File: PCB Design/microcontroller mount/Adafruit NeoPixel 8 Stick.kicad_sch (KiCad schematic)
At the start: 2 parts, among them CN2 1X4SMT, U1 DFR0282

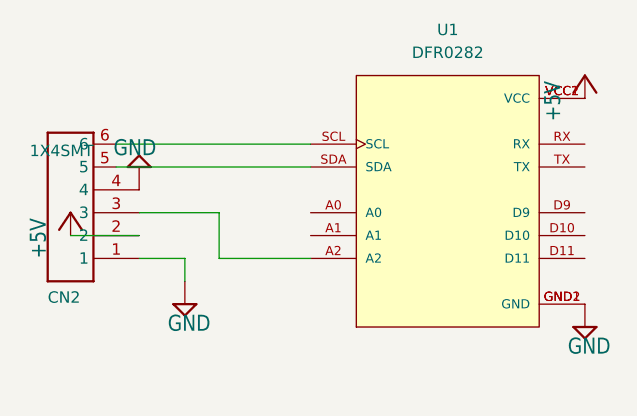
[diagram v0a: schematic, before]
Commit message: updates
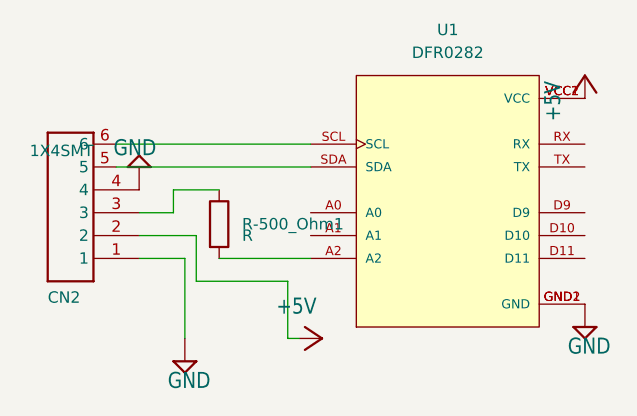
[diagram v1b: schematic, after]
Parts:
- added R-500_Ohm1: R, Resistor_THT:R_Axial_DIN0204_L3.6mm_D1.6mm_P7.62mm_Horizontal, symbol Device:R
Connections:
- net at CN2.3: now also R-500_Ohm1.1; no longer U1.A2
- new net: R-500_Ohm1.2, U1.A2
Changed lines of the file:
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@@
 (kicad_sch (version 20211123) (generator eeschema)
   (paper "A4")
+  (wire (pts (xy 46.99 129.54) (xy 57.15 129.54))
+    (stroke (width 0) (type default) (color 0 0 0 0))
+  )
   (wire (pts (xy 40.64 127) (xy 45.72 127))
     (stroke (width 0) (type default) (color 0 0 0 0))
   )
-  (wire (pts (xy 45.72 127) (xy 45.72 129.54))
-    (stroke (width 0) (type default) (color 0 0 0 0))
-  )
   (wire (pts (xy 38.1 116.84) (xy 59.69 116.84))
     (stroke (width 0) (type default) (color 0 0 0 0))
   )
+  (wire (pts (xy 44.45 119.38) (xy 44.45 121.92))
+    (stroke (width 0) (type default) (color 0 0 0 0))
+  )
+  (wire (pts (xy 49.53 119.38) (xy 44.45 119.38))
+    (stroke (width 0) (type default) (color 0 0 0 0))
+  )
   (wire (pts (xy 38.1 114.3) (xy 59.69 114.3))
     (stroke (width 0) (type default) (color 0 0 0 0))
   )
-  (wire (pts (xy 49.53 121.92) (xy 40.64 121.92))
-    (stroke (width 0) (type default) (color 0 0 0 0))
-  )
-  (wire (pts (xy 49.53 127) (xy 49.53 121.92))
-    (stroke (width 0) (type default) (color 0 0 0 0))
-  )
-  (wire (pts (xy 59.69 127) (xy 49.53 127))
-    (stroke (width 0) (type default) (color 0 0 0 0))
-  )
-  (wire (pts (xy 33.02 124.46) (xy 40.64 124.46))
+  (wire (pts (xy 49.53 127) (xy 59.69 127))
+    (stroke (width 0) (type default) (color 0 0 0 0))
+  )
+  (wire (pts (xy 46.99 124.46) (xy 46.99 129.54))
+    (stroke (width 0) (type default) (color 0 0 0 0))
+  )
+  (wire (pts (xy 45.72 127) (xy 45.72 135.89))
+    (stroke (width 0) (type default) (color 0 0 0 0))
+  )
+  (wire (pts (xy 57.15 135.89) (xy 58.42 135.89))
+    (stroke (width 0) (type default) (color 0 0 0 0))
+  )
+  (wire (pts (xy 57.15 129.54) (xy 57.15 135.89))
+    (stroke (width 0) (type default) (color 0 0 0 0))
+  )
+  (wire (pts (xy 44.45 121.92) (xy 40.64 121.92))
+    (stroke (width 0) (type default) (color 0 0 0 0))
+  )
+  (wire (pts (xy 40.64 124.46) (xy 46.99 124.46))
     (stroke (width 0) (type default) (color 0 0 0 0))
   )
@@
     (pin "1")
   )
+  (symbol (lib_id "Device:R") (at 49.53 123.19 0) (unit 1)
+    (in_bom yes) (on_board yes)
+    (property "Reference" "R-500_Ohm1" (id 0) (at 52.07 123.19 0)
+      (effects (font (size 1.27 1.27)) (justify left))
+    )
+    (property "Value" "R" (id 1) (at 52.07 124.4599 0)
+      (effects (font (size 1.27 1.27)) (justify left))
+    )
+    (property "Footprint" "Resistor_THT:R_Axial_DIN0204_L3.6mm_D1.6mm_P7.62mm_Horizontal" (id 2) (at 47.752 123.19 90)
+      (effects (font (size 1.27 1.27)) hide)
+    )
+    (property "Datasheet" "~" (id 3) (at 49.53 123.19 0)
+      (effects (font (size 1.27 1.27)) hide)
+    )
+    (pin "1")
+    (pin "2")
+  )
   (symbol (lib_id "Adafruit NeoPixel 8 Stick-eagle-import:GND") (at 40.64 116.84 180) (unit 1)
     (in_bom yes) (on_board yes)
@@
     (pin "1")
   )
-  (symbol (lib_id "Adafruit NeoPixel 8 Stick-eagle-import:+5V") (at 33.02 121.92 0) (unit 1)
-    (in_bom yes) (on_board yes)
-    (property "Reference" "#P+011" (id 0) (at 33.02 121.92 0)
-      (effects (font (size 1.27 1.27)) hide)
-    )
-    (property "Value" "+5V" (id 1) (at 30.48 127 90)
-      (effects (font (size 1.778 1.5113)) (justify left bottom))
-    )
-    (property "Footprint" "Adafruit NeoPixel 8 Stick:" (id 2) (at 33.02 121.92 0)
-      (effects (font (size 1.27 1.27)) hide)
-    )
-    (property "Datasheet" "" (id 3) (at 33.02 121.92 0)
-      (effects (font (size 1.27 1.27)) hide)
-    )
-    (pin "1")
-  )
-  (symbol (lib_id "Adafruit NeoPixel 8 Stick-eagle-import:GND") (at 45.72 132.08 0) (unit 1)
-    (in_bom yes) (on_board yes)
-    (property "Reference" "#SUPPLY07" (id 0) (at 45.72 132.08 0)
-      (effects (font (size 1.27 1.27)) hide)
-    )
-    (property "Value" "GND" (id 1) (at 43.815 135.255 0)
-      (effects (font (size 1.778 1.5113)) (justify left bottom))
-    )
-    (property "Footprint" "Adafruit NeoPixel 8 Stick:" (id 2) (at 45.72 132.08 0)
-      (effects (font (size 1.27 1.27)) hide)
-    )
-    (property "Datasheet" "" (id 3) (at 45.72 132.08 0)
+  (symbol (lib_id "Adafruit NeoPixel 8 Stick-eagle-import:+5V") (at 60.96 135.89 270) (unit 1)
+    (in_bom yes) (on_board yes)
+    (property "Reference" "#P+0102" (id 0) (at 60.96 135.89 0)
+      (effects (font (size 1.27 1.27)) hide)
+    )
+    (property "Value" "+5V" (id 1) (at 55.88 133.35 90)
+      (effects (font (size 1.778 1.5113)) (justify left bottom))
+    )
+    (property "Footprint" "Adafruit NeoPixel 8 Stick:" (id 2) (at 60.96 135.89 0)
+      (effects (font (size 1.27 1.27)) hide)
+    )
+    (property "Datasheet" "" (id 3) (at 60.96 135.89 0)
+      (effects (font (size 1.27 1.27)) hide)
+    )
+    (pin "1")
+  )
+  (symbol (lib_id "Adafruit NeoPixel 8 Stick-eagle-import:GND") (at 45.72 138.43 0) (unit 1)
+    (in_bom yes) (on_board yes)
+    (property "Reference" "#SUPPLY07" (id 0) (at 45.72 138.43 0)
+      (effects (font (size 1.27 1.27)) hide)
+    )
+    (property "Value" "GND" (id 1) (at 43.815 141.605 0)
+      (effects (font (size 1.778 1.5113)) (justify left bottom))
+    )
+    (property "Footprint" "Adafruit NeoPixel 8 Stick:" (id 2) (at 45.72 138.43 0)
+      (effects (font (size 1.27 1.27)) hide)
+    )
+    (property "Datasheet" "" (id 3) (at 45.72 138.43 0)
       (effects (font (size 1.27 1.27)) hide)
     )
@@
   )
   (symbol_instances
-    (path "/2200c74e-452f-432b-9f61-032e159036e1"
-      (reference "#P+011") (unit 1) (value "+5V") (footprint "Adafruit NeoPixel 8 Stick:")
-    )
     (path "/16106da6-22cc-43d0-bd4c-67ef6ba38d61"
       (reference "#P+0101") (unit 1) (value "+5V") (footprint "Adafruit NeoPixel 8 Stick:")
     )
+    (path "/37ba77a5-6ca2-4fbe-a6d2-b4abdc4b9fc5"
+      (reference "#P+0102") (unit 1) (value "+5V") (footprint "Adafruit NeoPixel 8 Stick:")
+    )
     (path "/14c3df3c-70c6-4ca9-a9fe-754465985686"
       (reference "#SUPPLY02") (unit 1) (value "GND") (footprint "Adafruit NeoPixel 8 Stick:")
@@
       (reference "CN2") (unit 1) (value "1X4SMT") (footprint "Adafruit NeoPixel 8 Stick:1X4-SMT")
     )
+    (path "/0cbfcb3d-71ff-4eea-9289-dea41a73539f"
+      (reference "R-500_Ohm1") (unit 1) (value "R") (footprint "Resistor_THT:R_Axial_DIN0204_L3.6mm_D1.6mm_P7.62mm_Horizontal")
+    )
     (path "/58301483-f474-4e36-8969-9e03af126b0a"
